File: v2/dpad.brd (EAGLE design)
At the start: 30 x 30.8 mm, 9 parts

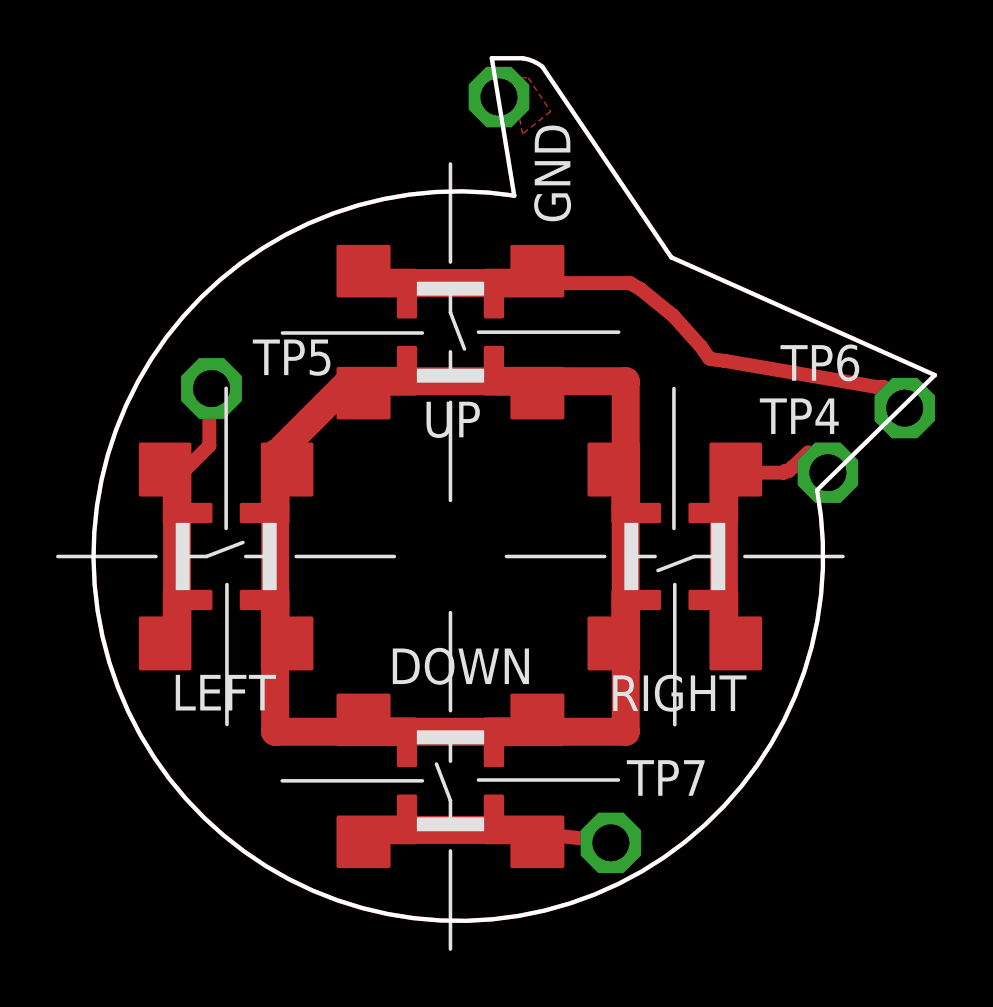
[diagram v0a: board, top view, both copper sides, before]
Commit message: Update to v2.1
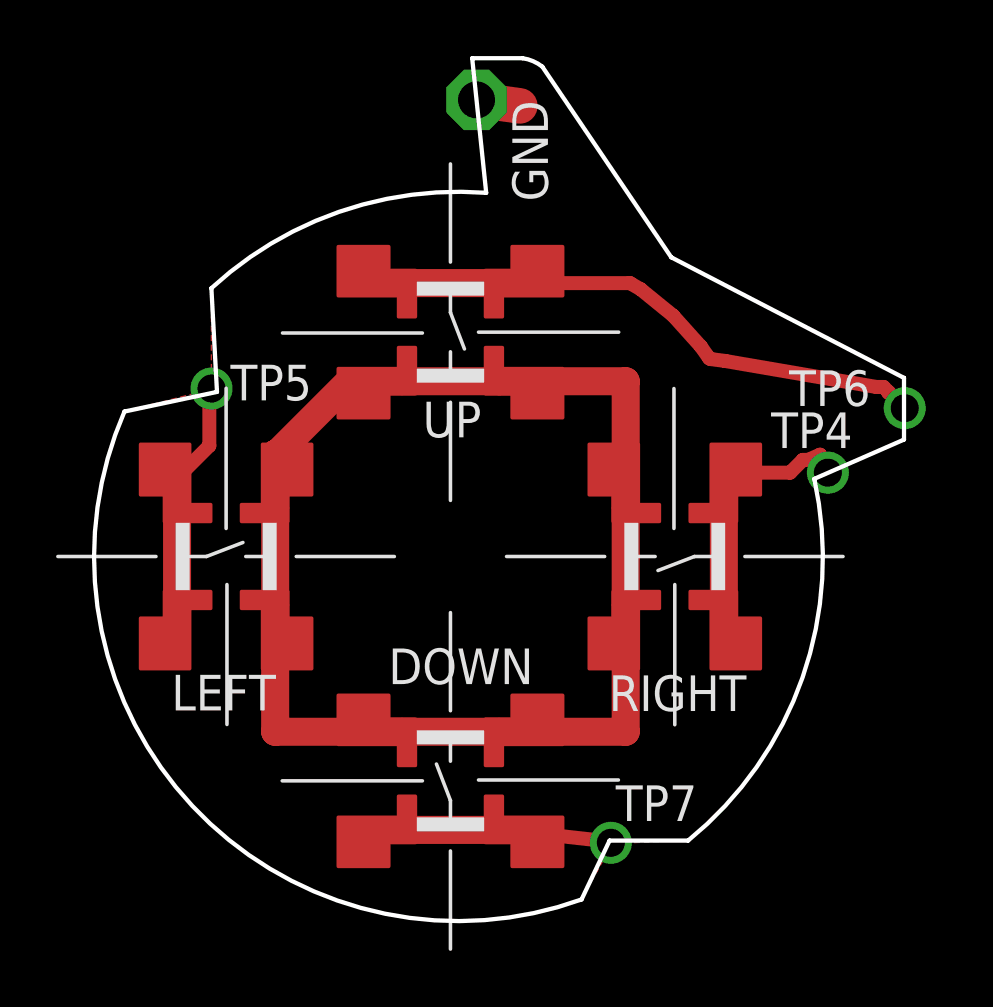
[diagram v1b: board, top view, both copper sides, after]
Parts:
- TP4, TP5, TP6, TP7: value TPPAD1-13 -> TESTPAD; device testpad:P1-13 -> lib:TESTPAD
- moved GND 0.81 mm to (14.5, 32.5)
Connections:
- net N$1: now also TP6.P$1; no longer TP6.TP
- net N$2: now also TP5.P$1; no longer TP5.TP
- net N$3: now also TP4.P$1; no longer TP4.TP
- net N$4: now also TP7.P$1; no longer TP7.TP
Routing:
- net GND: track 96.3 -> 51.6 mm
- net N$3: track 8.02 -> 9.07 mm
- net N$1: track 18.7 -> 19.5 mm
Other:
- board size 30 x 30.8 mm -> 28.9 x 30.8 mm
- board text added: "AGB_TACT_dpad_V2.1"
- board text removed: "AGB_TACT_dpad_V2.0"
